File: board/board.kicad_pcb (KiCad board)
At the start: 2 copper layers, 21 x 13 mm, 1 part

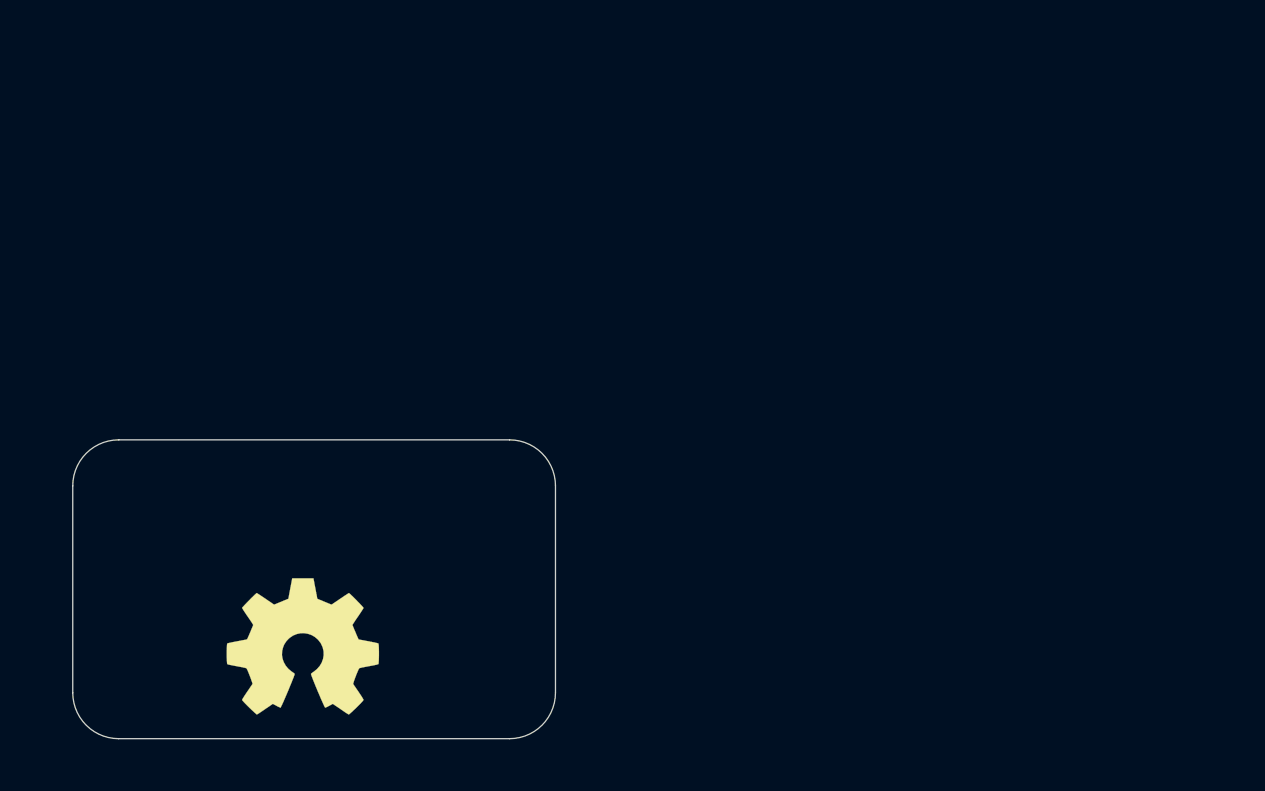
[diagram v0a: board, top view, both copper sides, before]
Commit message: initial
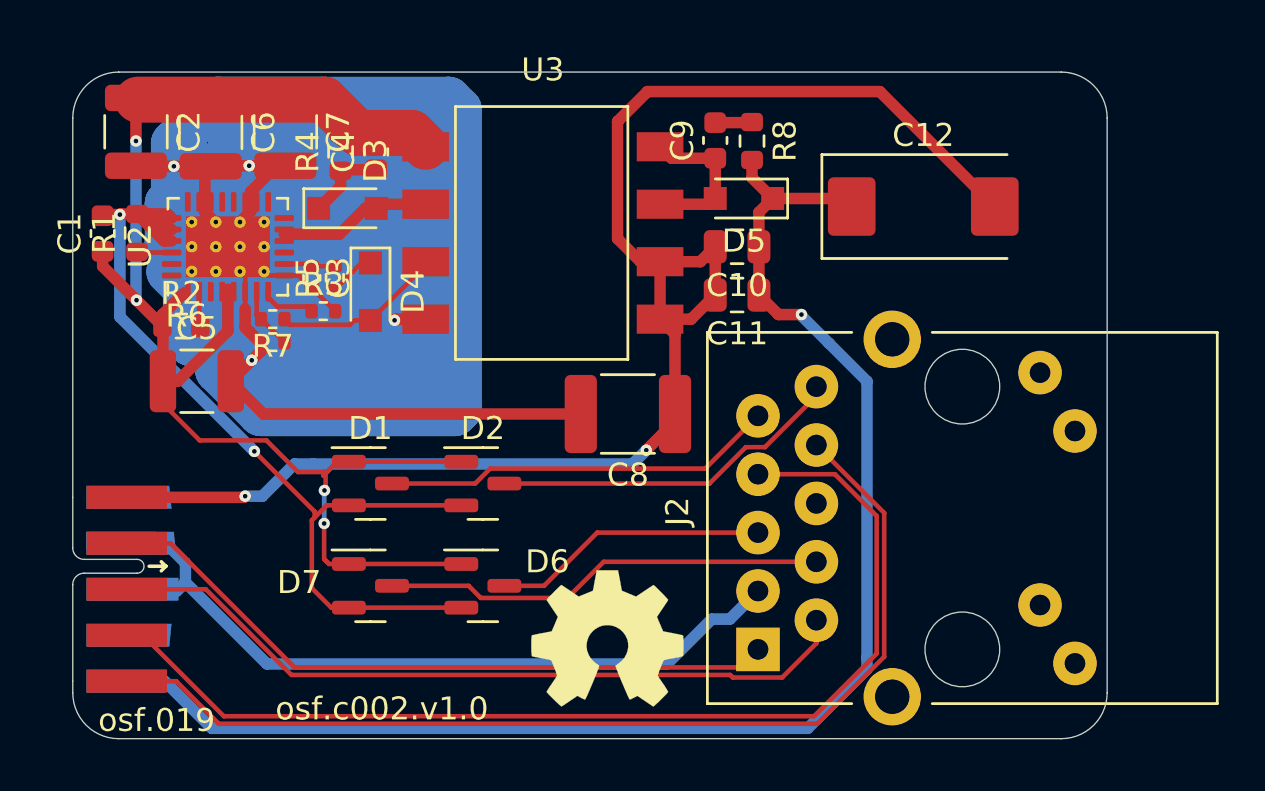
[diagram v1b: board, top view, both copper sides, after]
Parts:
- added C1: 100n, Capacitor_SMD:C_0603_1608Metric, F.Cu at (141.3, 81.0)
- added C10: 22uF, Capacitor_SMD:C_0805_2012Metric, F.Cu at (168.9, 81.6)
- added C11: 22uF, Capacitor_SMD:C_0805_2012Metric, F.Cu at (168.9, 83.7)
- added C12: 220u, Capacitor_Tantalum_SMD:CP_EIA-7343-31_Kemet-D, F.Cu at (177.0, 79.8)
- added C2: 2.2uF, Capacitor_SMD:C_1210_3225Metric, F.Cu at (142.8, 76.6)
- added C3: 100nF, Capacitor_SMD:C_0402_1005Metric, F.Cu at (150.4, 83.0)
- added C4: 10nF, Capacitor_SMD:C_0603_1608Metric, F.Cu at (153.2, 77.5)
- added C5: 2.2uF, Capacitor_SMD:C_1210_3225Metric, F.Cu at (145.4, 87.5)
- added C6: 2.2uF, Capacitor_SMD:C_1210_3225Metric, F.Cu at (146.0, 76.6)
- added C7: 2.2uF, Capacitor_SMD:C_1210_3225Metric, F.Cu at (149.2, 76.6)
- added C8: 1nF, Capacitor_SMD:C_1812_4532Metric, F.Cu at (164.2, 88.9)
- added C9: 10n, Capacitor_SMD:C_0603_1608Metric, F.Cu at (167.9, 77.0)
- added D1: BAV99, Package_TO_SOT_SMD:SOT-23, F.Cu at (152.9, 91.9)
- added D2: BAV99, Package_TO_SOT_SMD:SOT-23, F.Cu at (157.8, 91.9)
- added D3: BAV21WS-HE3-18, Diode_SMD:D_SOD-323_HandSoldering, F.Cu at (151.9, 79.9)
- added D4: 1N4148, Diode_SMD:D_SOD-323_HandSoldering, F.Cu at (152.9, 83.5)
- added D5: CUS15S30,H3F, Diode_SMD:D_SOD-323_HandSoldering, F.Cu at (169.2, 79.5)
- added D6: BAV99, Package_TO_SOT_SMD:SOT-23, F.Cu at (157.8, 96.3)
- added D7: BAV99, Package_TO_SOT_SMD:SOT-23, F.Cu at (152.9, 96.3)
- added J1: 019_100BASE-T_with_CT, on_edge:on_edge_2x05_device, F.Cu at (140.0, 96.5)
- added J2: LPJ4265BDNL, b135:LPJ4265BDNL, F.Cu at (169.8, 99.1)
- added R1: 41.2R, Resistor_SMD:R_0603_1608Metric, F.Cu at (142.8, 81.0)
- added R2: 24.9k, Resistor_SMD:R_0603_1608Metric, F.Cu at (144.7, 85.0)
- added R3: 100k, Resistor_SMD:R_0402_1005Metric, F.Cu at (150.9, 84.4)
- added R4: 10k, Resistor_SMD:R_0603_1608Metric, F.Cu at (151.7, 77.5)
- added R5: 5k, Resistor_SMD:R_0402_1005Metric, F.Cu at (151.4, 83.0)
- added R6: 20k, Resistor_SMD:R_0402_1005Metric, F.Cu at (148.7, 85.8)
- added R7: 100k, Resistor_SMD:R_0402_1005Metric, F.Cu at (148.7, 84.8)
- added R8: 20R, Resistor_SMD:R_0603_1608Metric, F.Cu at (169.6, 77.0)
- added U2: MP8007, Package_DFN_QFN:QFN-28-1EP_4x5mm_P0.5mm_EP2.65x3.65mm_ThermalVias, F.Cu at (146.8, 81.6)
- added U3: POE30P-50L, b033:Transformer_Coilcraft_POE30P, F.Cu at (160.4, 81.0)
- moved LOGO1 13.3 mm to (163.2, 98.7)
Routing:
- net /Controller/GNDPWR: track 0.00 -> 196.7 mm, vias 0 -> 4
- net GND: track 0.00 -> 66.4 mm, vias 0 -> 2
- net /Controller/5V: track 0.00 -> 63.1 mm, vias 0 -> 1
- net /Controller/PoE+: track 0.00 -> 63.0 mm, vias 0 -> 4
- net /magjack/RX+: track 0.00 -> 47.1 mm
- net /magjack/RX-: track 0.00 -> 45.4 mm
- net /Controller/PoE-: track 0.00 -> 40.1 mm, vias 0 -> 2
- net /magjack/CT: track 0.00 -> 34.2 mm
- net /magjack/TX-: track 0.00 -> 33.2 mm
- net /magjack/TX+: track 0.00 -> 30.0 mm
- net /magjack/CT4: track 0.00 -> 19.3 mm
- net /magjack/CT1: track 0.00 -> 17.1 mm
- net /magjack/CT2: track 0.00 -> 15.5 mm
- net /magjack/CT3: track 0.00 -> 12.0 mm
- net Net-(D4-Pad2): track 0.00 -> 7.47 mm
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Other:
- board size 21 x 13 mm -> 45 x 29 mm
- board text added: "osf.019"
- board text added: "osf.c002.v1.0"
